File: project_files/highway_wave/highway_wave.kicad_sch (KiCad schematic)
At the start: 2 parts, among them U1 RASPBERRY_PI_ZERO_2_W, U2 GW1N-LV9QN88C6_I5_

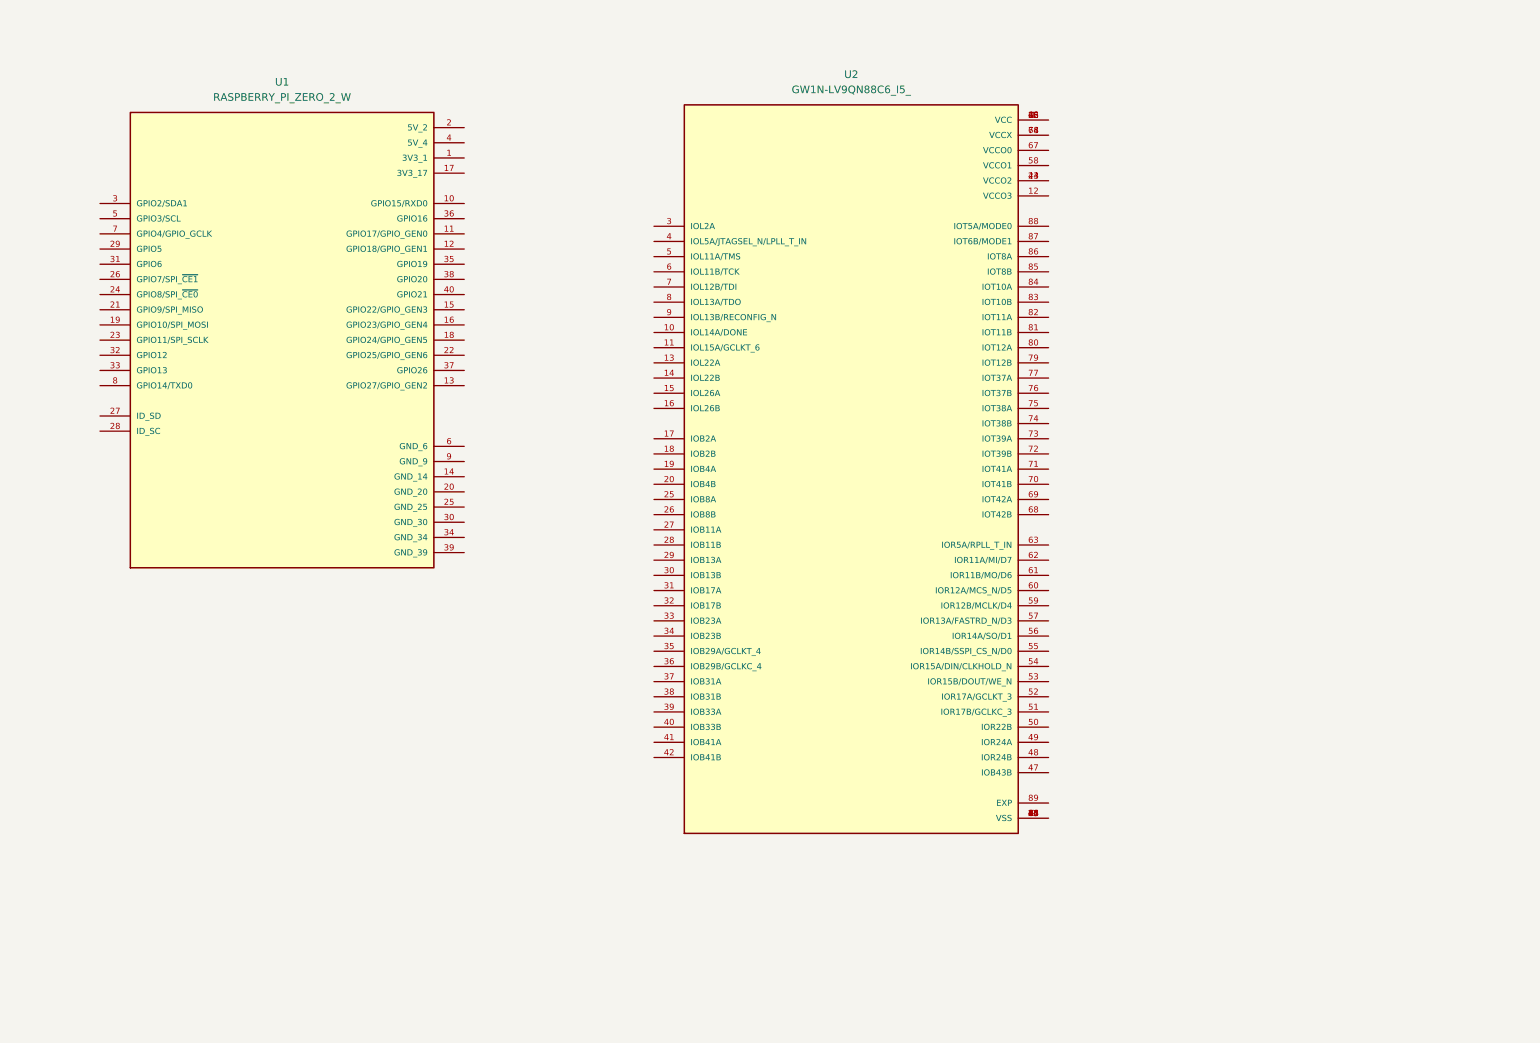
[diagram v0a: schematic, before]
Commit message: finished schem
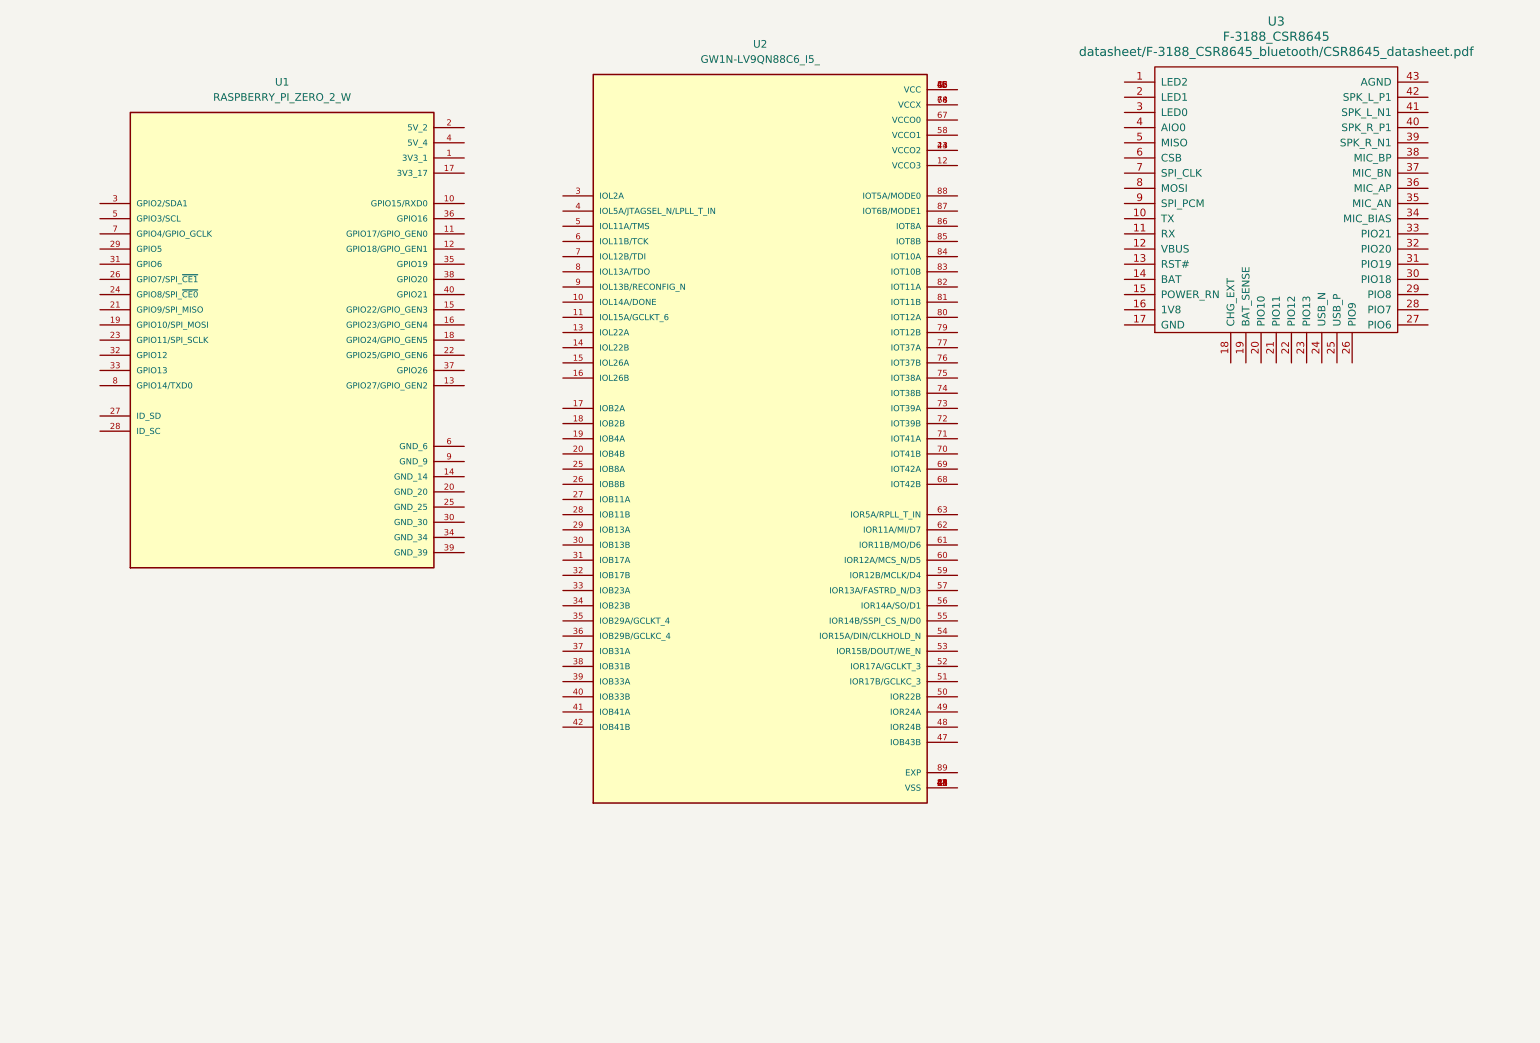
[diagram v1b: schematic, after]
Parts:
- added U3: F-3188_CSR8645, symbol F-3188_CSR8645:F-3188_CSR8645
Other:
- moved on the sheet: U2
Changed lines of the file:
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@@
+	)
+	(symbol
+		(lib_id "F-3188_CSR8645:F-3188_CSR8645")
+		(at 243.84 68.58 0)
+		(unit 1)
+		(exclude_from_sim no)
+		(in_bom yes)
+		(on_board yes)
+		(dnp no)
+		(fields_autoplaced yes)
+		(property "Reference" "U3"
+			(at 238.76 19.05 0)
+			(effects
+				(font
+					(size 1.524 1.524)
+				)
+			)
+		)
+		(property "Value" "F-3188_CSR8645"
+			(at 238.76 21.59 0)
+			(effects
+				(font
+					(size 1.524 1.524)
+				)
+			)
+		)
+		(property "Footprint" ""
+			(at 243.84 111.76 0)
+			(effects
+				(font
+					(size 1.524 1.524)
+				)
+			)
+		)
+		(property "Datasheet" "datasheet/F-3188_CSR8645_bluetooth/CSR8645_datasheet.pdf"
+			(at 238.76 24.13 0)
+			(effects
+				(font
+					(size 1.524 1.524)
+				)
+			)
+		)
+		(property "Description" ""
+			(at 243.84 68.58 0)
+			(effects
+				(font
+					(size 1.27 1.27)
+				)
+				(hide yes)
+			)
+		)
+		(pin "23"
+		)
+		(pin "24"
+		)
+		(pin "16"
+		)
+		(pin "32"
+		)
+		(pin "1"
+		)
+		(pin "21"
+		)
+		(pin "27"
+		)
+		(pin "29"
+		)
+		(pin "11"
+		)
+		(pin "2"
+		)
+		(pin "25"
+		)
+		(pin "15"
+		)
+		(pin "37"
+		)
+		(pin "3"
+		)
+		(pin "39"
+		)
+		(pin "4"
+		)
+		(pin "41"
+		)
+		(pin "28"
+		)
+		(pin "30"
+		)
+		(pin "22"
+		)
+		(pin "31"
+		)
+		(pin "10"
+		)
+		(pin "34"
+		)
+		(pin "12"
+		)
+		(pin "13"
+		)
+		(pin "17"
+		)
+		(pin "36"
+		)
+		(pin "14"
+		)
+		(pin "40"
+		)
+		(pin "20"
+		)
+		(pin "43"
+		)
+		(pin "5"
+		)
+		(pin "35"
+		)
+		(pin "19"
+		)
+		(pin "6"
+		)
+		(pin "7"
+		)
+		(pin "26"
+		)
+		(pin "18"
+		)
+		(pin "33"
+		)
+		(pin "8"
+		)
+		(pin "9"
+		)
+		(pin "38"
+		)
+		(pin "42"
+		)
+		(instances
+			(project ""
+				(path "/4d93a0f5-0323-4b77-816b-e07a1b9b3cd9"
+					(reference "U3")
+					(unit 1)
+				)
+			)
+		)
 	)
 	(symbol
 		(lib_id "GW1N-LV9QN88C6_I5_:GW1N-LV9QN88C6_I5_")
-		(at 167.64 93.98 0)
+		(at 152.4 88.9 0)
 		(unit 1)
 		(exclude_from_sim no)
@@
 		(fields_autoplaced yes)
 		(property "Reference" "U2"
-			(at 167.64 27.94 0)
+			(at 152.4 22.86 0)
 			(effects
 				(font
@@
 		)
 		(property "Value" "GW1N-LV9QN88C6_I5_"
-			(at 167.64 30.48 0)
+			(at 152.4 25.4 0)
 			(effects
 				(font
@@
 		)
 		(property "Footprint" "GW1N-LV9QN88C6_I5_:QFN40P1000X1000X95-89N"
-			(at 167.64 93.98 0)
+			(at 152.4 88.9 0)
 			(effects
 				(font
@@
 		)
 		(property "Datasheet" ""
-			(at 167.64 93.98 0)
+			(at 152.4 88.9 0)
 			(effects
 				(font
@@
 		)
 		(property "Description" ""
-			(at 167.64 93.98 0)
+			(at 152.4 88.9 0)
 			(effects
 				(font
@@
 		)
 		(property "MF" "Gowin Semiconductor"
-			(at 167.64 93.98 0)
+			(at 152.4 88.9 0)
 			(effects
 				(font
@@
 		)
 		(property "Description_1" "\n                        \n                            Volatile SRAM based and non-volatile flash-based field-programmable gate array (FPGA) technology\n                        \n"
-			(at 167.64 93.98 0)
+			(at 152.4 88.9 0)
 			(effects
 				(font
@@
 		)
 		(property "Package" "Package"
-			(at 167.64 93.98 0)
+			(at 152.4 88.9 0)
 			(effects
 				(font
@@
 		)
 		(property "Price" "None"
-			(at 167.64 93.98 0)
+			(at 152.4 88.9 0)
 			(effects
 				(font
@@
 		)
 		(property "Check_prices" "https://www.snapeda.com/parts/GW1N-LV9QN88C6/I5//Gowin+Semiconductor/view-part/?ref=eda"
-			(at 167.64 93.98 0)
+			(at 152.4 88.9 0)
 			(effects
 				(font
@@
 		)
 		(property "MAXIMUM_PACKAGE_HIEGHT" "0.95mm"
-			(at 167.64 93.98 0)
+			(at 152.4 88.9 0)
 			(effects
 				(font
@@
 		)
 		(property "STANDARD" "IPC7351B"
-			(at 167.64 93.98 0)
+			(at 152.4 88.9 0)
 			(effects
 				(font
@@
 		)
 		(property "PARTREV" "UG103-2.3E"
-			(at 167.64 93.98 0)
+			(at 152.4 88.9 0)
 			(effects
 				(font
@@
 		)
 		(property "SnapEDA_Link" "https://www.snapeda.com/parts/GW1N-LV9QN88C6/I5//Gowin+Semiconductor/view-part/?ref=snap"
-			(at 167.64 93.98 0)
+			(at 152.4 88.9 0)
 			(effects
 				(font
@@
 		)
 		(property "MP" "GW1N-LV9QN88C6/I5/"
-			(at 167.64 93.98 0)
+			(at 152.4 88.9 0)
 			(effects
 				(font
@@
 		)
 		(property "Availability" "In Stock"
-			(at 167.64 93.98 0)
+			(at 152.4 88.9 0)
 			(effects
 				(font
@@
 		)
 		(property "MANUFACTURER" "Gowin Semiconductor"
-			(at 167.64 93.98 0)
-			(effects
-				(font
+			(at 152.4 88.9 0)
+			(effects
+				(font

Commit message: exported schem
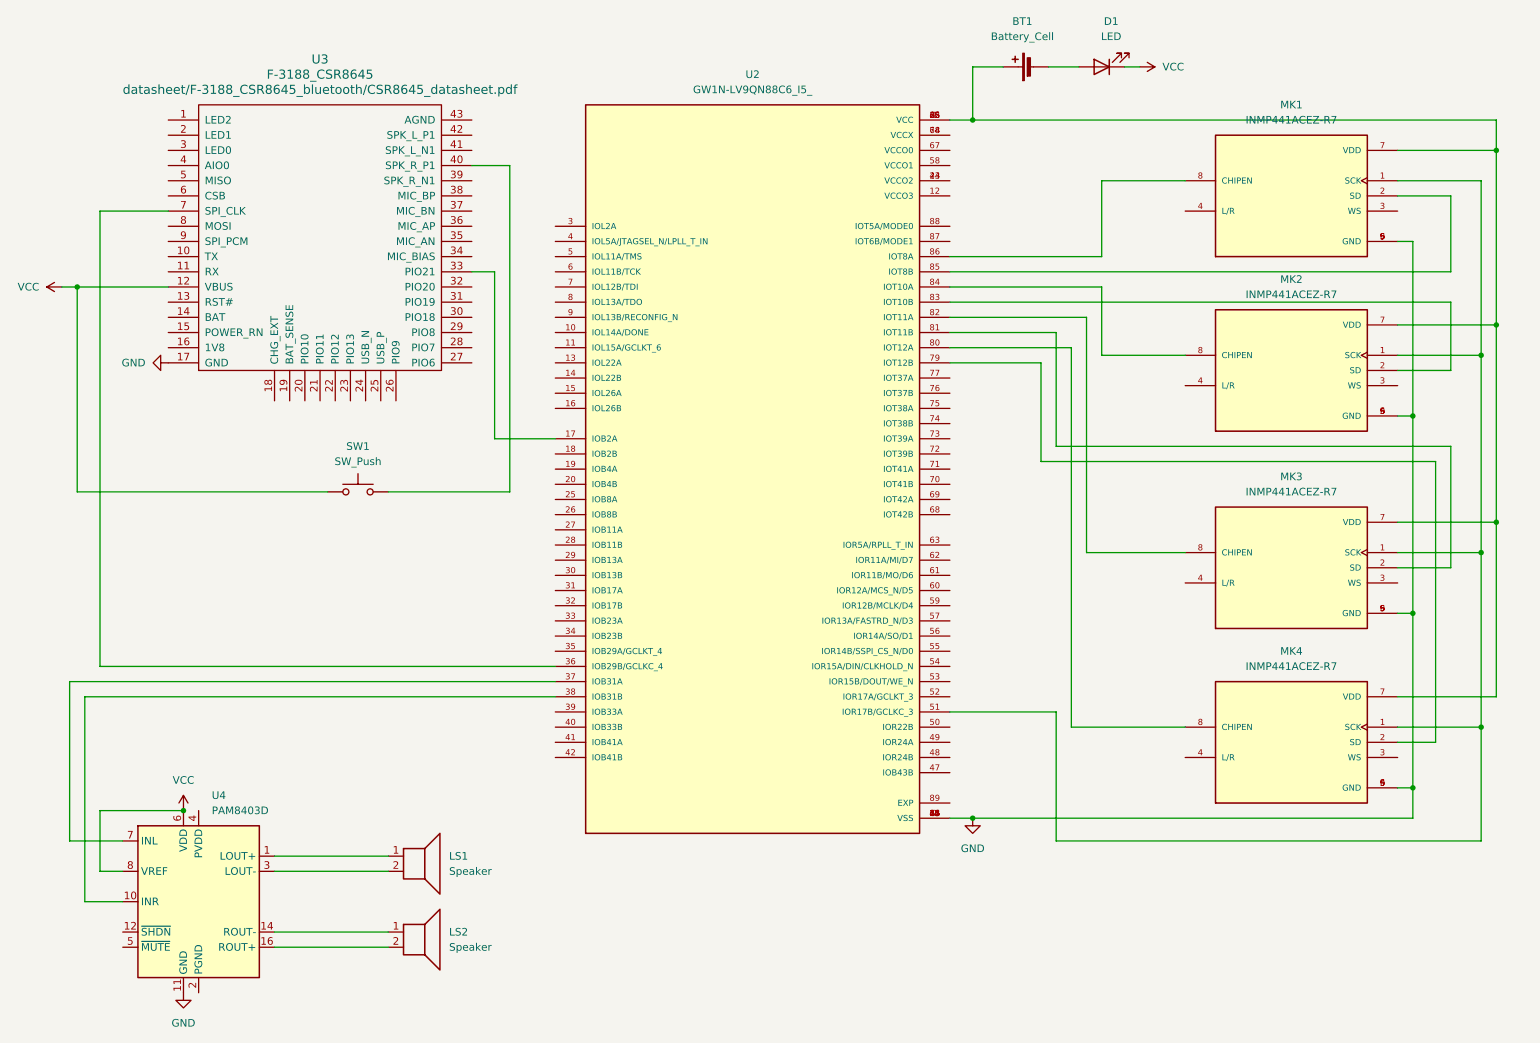
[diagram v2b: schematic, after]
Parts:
- removed U1: RASPBERRY_PI_ZERO_2_W, RASPBERRY_PI_ZERO_2_W:MODULE_RASPBERRY_PI_ZERO_2_W, symbol RASPBERRY_PI_ZERO_2_W:RASPBERRY_PI_ZERO_2_W
- added BT1: Battery_Cell, symbol Device:Battery_Cell
- added D1: LED, symbol Device:LED
- added LS1, LS2: Speaker, symbol Device:Speaker
- added MK1, MK2, MK3, MK4: INMP441ACEZ-R7, INMP441ACEZ-R7:MIC_INMP441ACEZ-R7, symbol INMP441ACEZ-R7:INMP441ACEZ-R7
- added SW1: SW_Push, symbol Switch:SW_Push
- added U4: PAM8403D, Package_SO:SOP-16_3.9x9.9mm_P1.27mm, symbol Amplifier_Audio:PAM8403D
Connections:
- net VCC: now reaches U3.12 (VBUS)
- net VCC: now also D1.1 (K), SW1.1, U4.6 (VDD), U4.8 (VREF)
- net GND: now reaches U3.17 (GND)
- net GND: now also U2.2 (VSS), U2.21 (VSS), U2.24 (VSS), U2.43 (VSS), U2.46 (VSS), U2.65 (VSS), MK1.5 (GND), MK1.6 (GND), MK1.9 (GND), MK2.5 (GND), MK2.6 (GND), MK2.9 (GND), MK3.5 (GND), MK3.6 (GND), MK3.9 (GND), MK4.5 (GND), MK4.6 (GND), MK4.9 (GND), U4.11 (GND)
- net at U3.33 (PIO21): now also U2.17 (IOB2A)
- net at U3.40 (SPK_R_P1): now also SW1.2
- net at U3.7 (SPI_CLK): now also U2.36 (IOB29B/GCLKC_4)
- net at U2.1 (VCC), U2.22 (VCC), U2.45 (VCC)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: now also BT1.1 (+), MK1.7 (VDD), MK2.7 (VDD), MK3.7 (VDD), MK4.7 (VDD)
- net at U2.37 (IOB31A): now also U4.7 (INL)
- net at U2.38 (IOB31B): now also U4.10 (INR)
- net at U2.51 (IOR17B/GCLKC_3): now also MK1.1 (SCK), MK2.1 (SCK), MK3.1 (SCK), MK4.1 (SCK)
- net at U2.79 (IOT12B): now also MK4.2 (SD)
- net at U2.80 (IOT12A): now also MK4.8 (CHIPEN)
- net at U2.81 (IOT11B): now also MK3.2 (SD)
- net at U2.82 (IOT11A): now also MK3.8 (CHIPEN)
- net at U2.83 (IOT10B): now also MK2.2 (SD)
- net at U2.84 (IOT10A): now also MK2.8 (CHIPEN)
- net at U2.85 (IOT8B): now also MK1.2 (SD)
- net at U2.86 (IOT8A): now also MK1.8 (CHIPEN)
- new net: BT1.2 (-), D1.2 (A)
- new net: LS2.1, U4.14 (ROUT-)
- new net: LS2.2, U4.16 (ROUT+)
- new net: LS1.1, U4.1 (LOUT+)
- new net: LS1.2, U4.3 (LOUT-)
- new net: U4.13 (PVDD), U4.4 (PVDD)
- new net: U4.15 (PGND), U4.2 (PGND)
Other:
- title: (none) -> Highway Wave
- moved on the sheet: U2, U3
